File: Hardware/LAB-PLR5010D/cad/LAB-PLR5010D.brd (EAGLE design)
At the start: 44.5 x 29.2 mm, 8 parts, among them J2 22-23-2021, J3 22-23-2021, U1 DAC8562, U2 LT3080, U3 LT3080

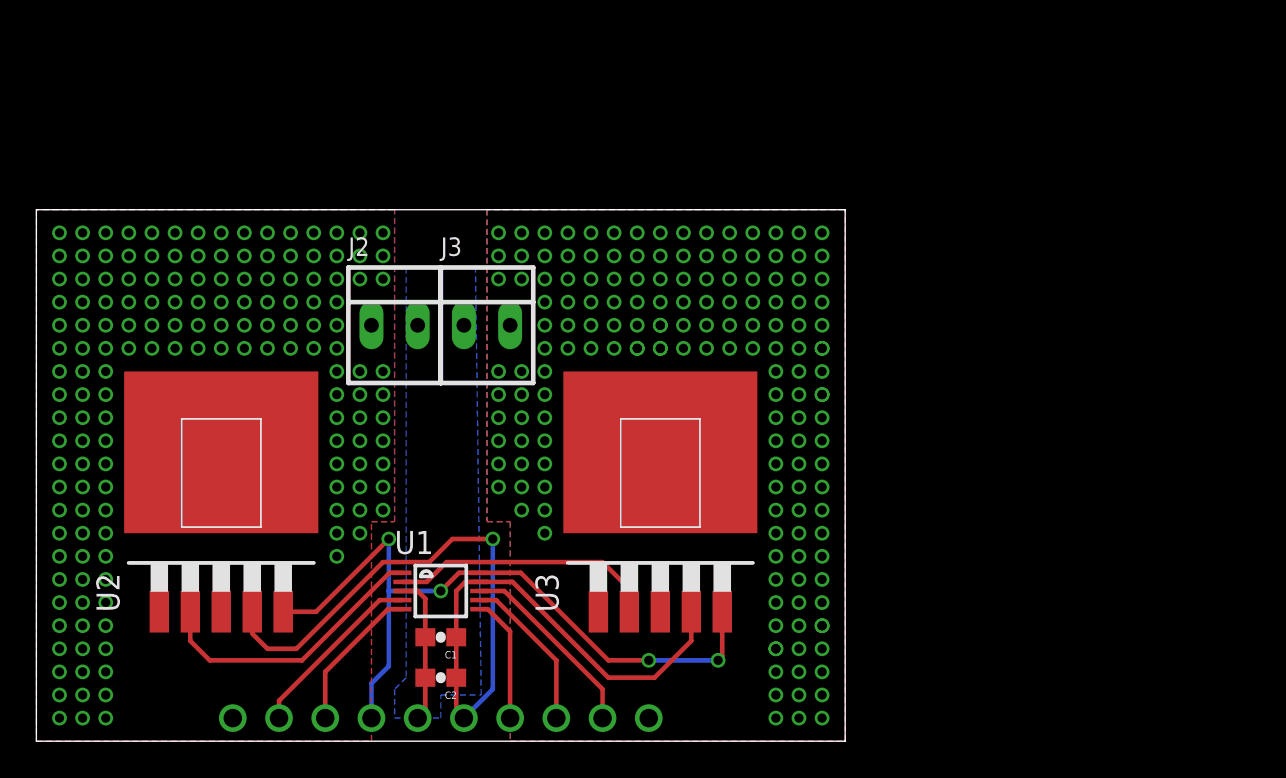
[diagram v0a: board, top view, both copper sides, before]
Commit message: 1) Committing final Rev0 of the PLR5010
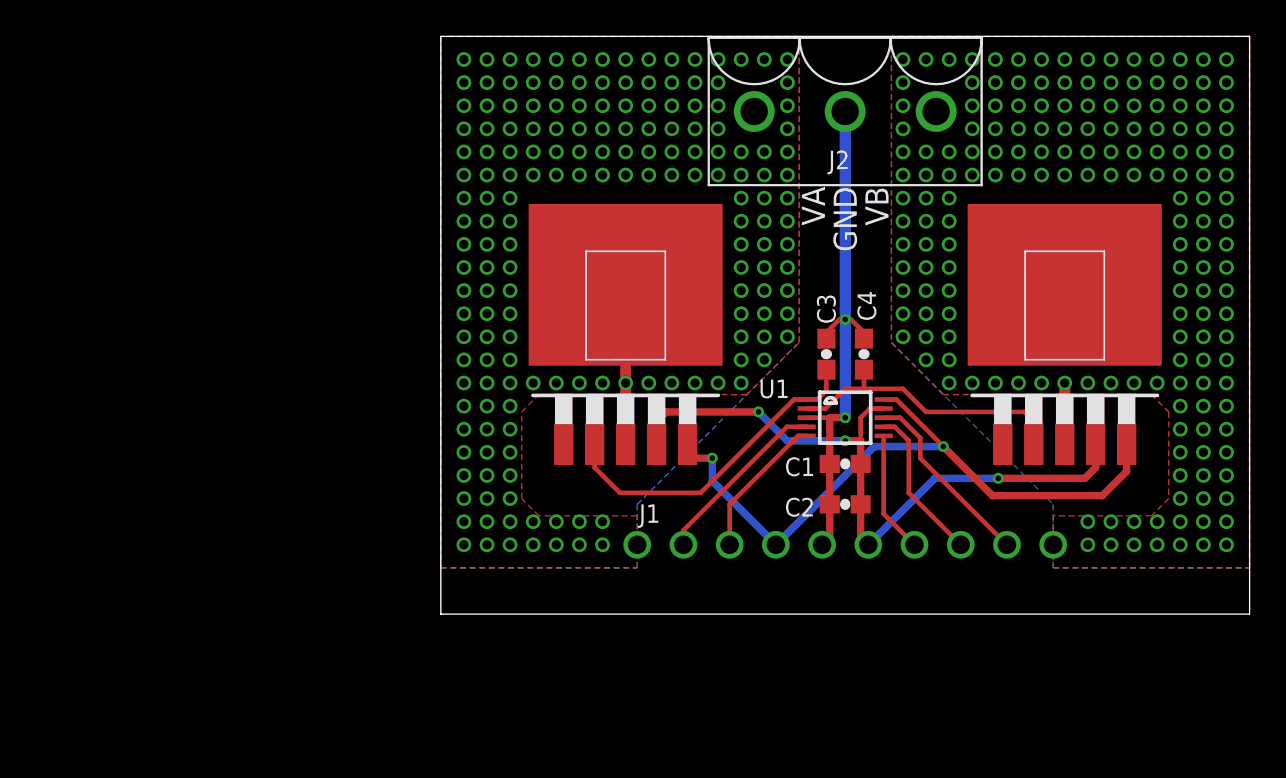
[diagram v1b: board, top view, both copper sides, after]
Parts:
- removed J3: 22-23-2021, My Library-adm:22-23-2021
- added C3, C4: 33nf, SparkFun-Capacitors:0603-CAP
- J2: value 22-23-2021 -> 1729021; device My Library-adm:22-23-2021 -> My Library-adm:1729021
- moved J2 27.4 mm to (22.2, 27.6)
- moved C1 24.2 mm to (22.2, 8.26)
- moved C2 24.2 mm to (22.2, 6.03)
- moved J1 24.2 mm to (22.2, 3.81)
- moved U1 24.2 mm to (22.2, 10.8)
- moved U2 24.1 mm to (10.2, 18.1)
- moved U3 24.1 mm to (34.3, 18.1)
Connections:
- net GND: now also C3.2, C4.2, J2.P$2; no longer J2.2, J3.1
- net N$2: now also C3.1
- net N$3: now also C4.1
- net VA: now also J2.P$1; no longer J2.1
- net VB: now also J2.P$3; no longer J3.2
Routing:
- net GND: track 8.18 -> 29.4 mm, vias 0 -> 2
- net VDDIO: track 52.7 -> 38.8 mm, vias 1 -> 3
- net VA: track 0.00 -> 8.76 mm, vias 156 -> 173
- net VDDLDO: track 41.0 -> 37.3 mm, vias 4 -> 2
- net VB: track 0.00 -> 3.37 mm, vias 160 -> 173
- net N$2: track 15.7 -> 18.1 mm
- net N$3: track 14.8 -> 16.0 mm
- removed copper zone on layer 16, net GND
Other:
- board size 44.5 x 29.2 mm -> 44.5 x 31.8 mm
- board text added: "!CLR"
- board text added: "!CS"
- board text added: "!LDAC"
- board text added: "GND"
- board text added: "LAB-PLR5010D"
- board text added: "MCLK"
- board text added: "MOSI"
- board text added: "VA"
- board text added: "VB"
- board text added: "VDDIO"
- board text added: "VDDLDO"

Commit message: 1) Checkpoint before cleanup, final BOM and MFG
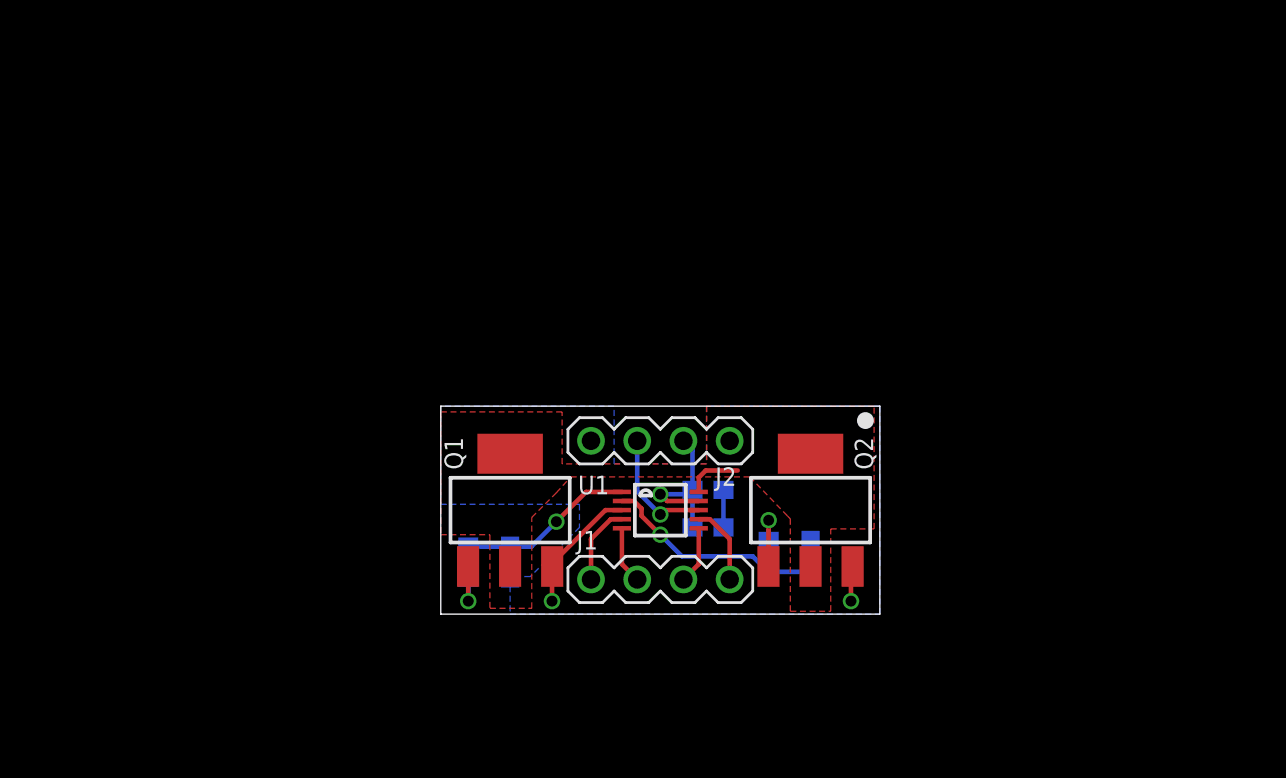
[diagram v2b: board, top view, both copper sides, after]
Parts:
- removed U2, U3: LT3080, LAB-PLR1010:DDPAK5(Q)
- added Q1, Q2: FZT849, LAB304:SOT223
- added R1, R2: (no value), rcl:R0603
- J1: device con-lstb:MA10-1W -> con-lstb:MA04-1
- J2: value 1729021 -> (none); device My Library-adm:1729021 -> con-lstb:MA04-1
- moved C3 20.8 mm to (3.81, 2.86), flipped to the bottom, turned to 270 degrees
- moved J2 20.8 mm to (12.1, 9.53)
- moved C4 11.5 mm to (20.3, 3.17), flipped to the bottom
- moved U1 11.4 mm to (12.1, 5.71)
- moved J1 10.3 mm to (12.1, 1.91), flipped to the top, turned to 0 degrees
- moved C1 7.67 mm to (14.7, 6.83), flipped to the bottom
- moved C2 7.65 mm to (14.7, 4.76), flipped to the bottom
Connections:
- removed net N$2: C3.1, U1.1, U2.2
- removed net VA: J1.1, J2.P$1, U2.3, U2.TAB
- removed net VB: J1.10, J2.P$3, U3.3, U3.TAB
- new net N$1: C3.1, R1.1, U1.1
- new net N$4: Q1.1, R1.2
- new net N$5: Q2.1, R2.2
- net !CLR: now also J1.2; no longer J1.3
- net !CS: now also J1.3; no longer J1.7
- net !LDAC: now also J1.1; no longer J1.2
- net GND: now also J2.1, Q1.3, Q2.3; no longer J1.5, J2.P$2
- net MCLK: now also J1.4; no longer J1.8
- net MOSI: now also J2.2; no longer J1.9
- net N$3: now also R2.1; no longer U3.2
- net VDDIO: now also J2.3; no longer J1.6, U2.4, U3.4
- net VDDLDO: now also J2.4, Q1.2, Q1.4, Q2.2, Q2.4; no longer J1.4, U2.5, U3.5
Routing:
- net VDDLDO: track 37.3 -> 3.31 mm, vias 2 -> 0
- net VDDIO: track 38.8 -> 9.11 mm, vias 3 -> 1
- net N$2: track 18.1 -> 0.00 mm
- net GND: track 29.4 -> 11.5 mm
- net N$1: track 0.00 -> 9.69 mm, vias 0 -> 1
- net VA: track 8.76 -> 0.00 mm, vias 173 -> 0
- net !LDAC: track 9.93 -> 4.37 mm
- net !CLR: track 8.02 -> 3.16 mm
- net MCLK: track 8.60 -> 4.37 mm
- net N$3: track 16.0 -> 12.2 mm, vias 0 -> 1
- net N$5: track 0.00 -> 3.75 mm, vias 0 -> 1
- net MOSI: track 10.3 -> 6.79 mm, vias 0 -> 1
- net !CS: track 6.69 -> 3.16 mm
- net VB: track 3.37 -> 0.00 mm, vias 173 -> 0
- net N$4: track 0.00 -> 3.22 mm, vias 0 -> 1
- added copper zone on layer 16, net GND
- added copper zone on layer 1, net VDDLDO
- removed copper zone on layer 1, net VA
- removed copper zone on layer 16, net VA
- removed copper zone on layer 1, net VB
- removed copper zone on layer 16, net VB
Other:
- board size 44.5 x 31.8 mm -> 24.1 x 11.4 mm
- board text added: "LAB-PLR"
- board text added: "PLR5010D"
- board text added: "VLDO"
- board text removed: "LAB-PLR5010D"
- board text removed: "VA"
- board text removed: "VB"
- board text removed: "VDDLDO"

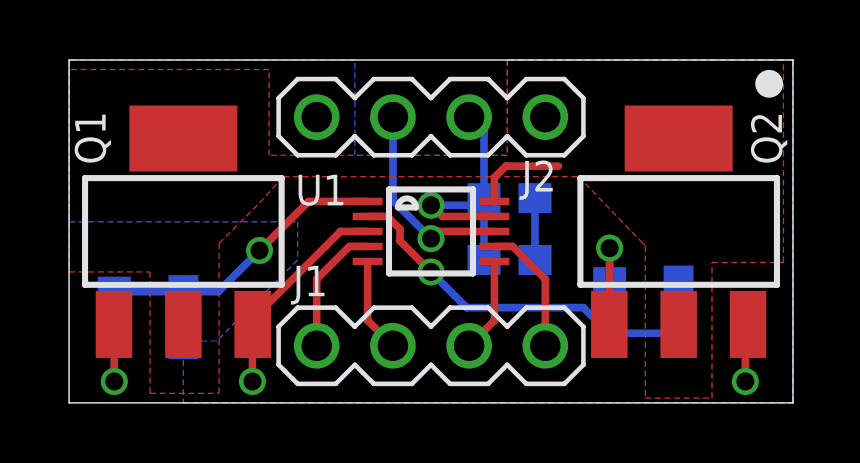
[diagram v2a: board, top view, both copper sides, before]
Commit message: 1) Releasing new revision for MFG
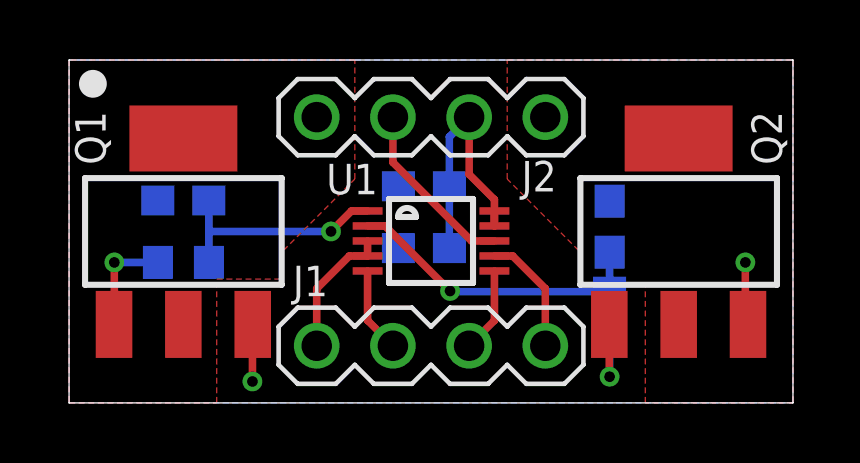
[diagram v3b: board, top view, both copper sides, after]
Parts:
- R1, R2: value (none) -> 390R
- U1: device LAB-PLR1010:MSOP10 -> LAB-PLR5010D:MSOP10
- moved C3 3.89 mm to (3.81, 6.75), turned to 0 degrees
- moved C4 3.55 mm to (18.0, 5.87)
- moved R1 2.94 mm to (3.81, 4.68), turned to 0 degrees
- moved C1 2.88 mm to (11.8, 7.22), turned to 0 degrees
- moved C2 2.88 mm to (11.8, 5.16), turned to 0 degrees
- moved R2 0.32 mm to (18.0, 2.86), turned to 270 degrees
- moved U1 0.32 mm to (12.1, 5.40)
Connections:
- removed net !LDAC: J1.1, U1.4
- removed net VDDIO: C1.1, C2.1, J2.3, U1.9
- removed net VDDLDO: J2.4, Q1.2, Q1.4, Q2.2, Q2.4, U1.10
- new net CHA: J2.1, Q1.2, Q1.4
- new net CHB: J2.4, Q2.2, Q2.4
- new net VDD: C1.1, C2.1, J2.3, U1.10, U1.9
- net GND: now also J1.1, U1.4; no longer J2.1
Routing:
- net VDD: track 0.00 -> 9.15 mm
- net VDDIO: track 9.11 -> 0.00 mm, vias 1 -> 0
- net !LDAC: track 4.37 -> 0.00 mm
- net VDDLDO: track 3.31 -> 0.00 mm
- net GND: track 11.5 -> 8.89 mm
- net N$1: track 9.69 -> 7.64 mm
- net N$3: track 12.2 -> 10.3 mm
- net N$4: track 3.22 -> 4.77 mm
- net N$5: track 3.75 -> 2.88 mm
- net MOSI: track 6.79 -> 5.98 mm, vias 1 -> 0
- added copper zone on layer 1, net CHA
- added copper zone on layer 1, net CHB
- removed copper zone on layer 1, net VDDLDO
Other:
- board text added: "CHA"
- board text added: "CHB"
- board text added: "VDD"
- board text removed: "!LDAC"
- board text removed: "VDDIO"
- board text removed: "VLDO"
